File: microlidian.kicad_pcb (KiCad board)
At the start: 2 copper layers, 148.7 x 128.5 mm, 31 parts, among them J1 Conn_02x05_Odd_Even, J11 Backboard Conn 1, J12 Frontboard Conn 1, J13 Backboard Conn 2, J14 Frontboard Conn 2, J2 ST7789 TFT socket, J3 Expansion header, J4 ADS1015 digital side, J5 ADS1015 analog side, J7 TRS MIDI Out, SW1 RotaryEncoder_Switch, SW2 Back button, U1 SeeeduinoXIAO, U2 L78L05_TO92

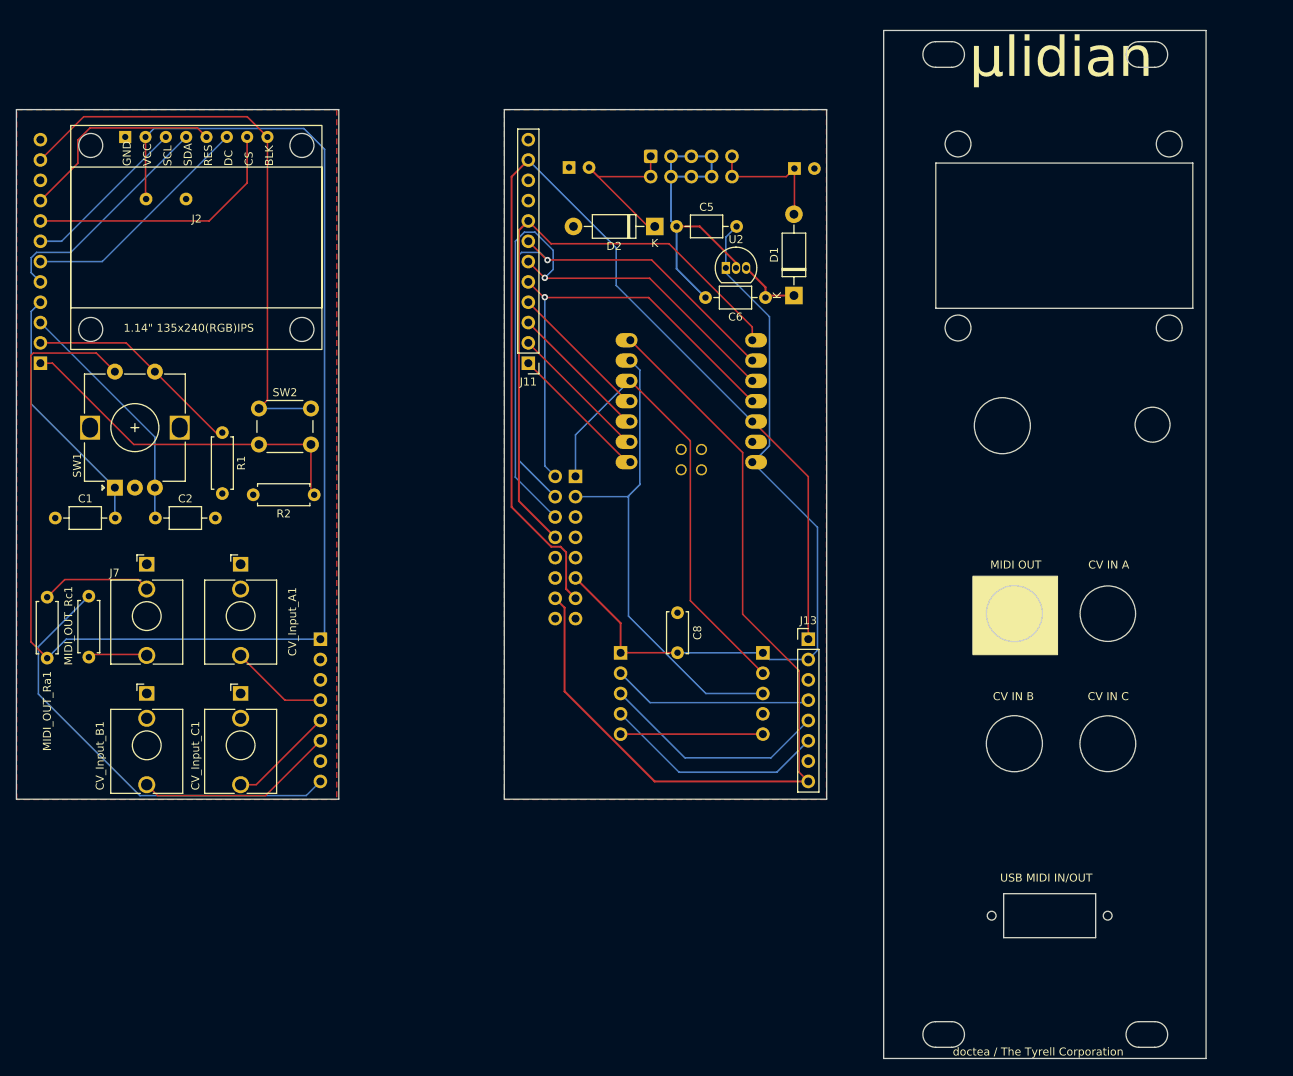
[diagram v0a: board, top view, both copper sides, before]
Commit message: some minor updates
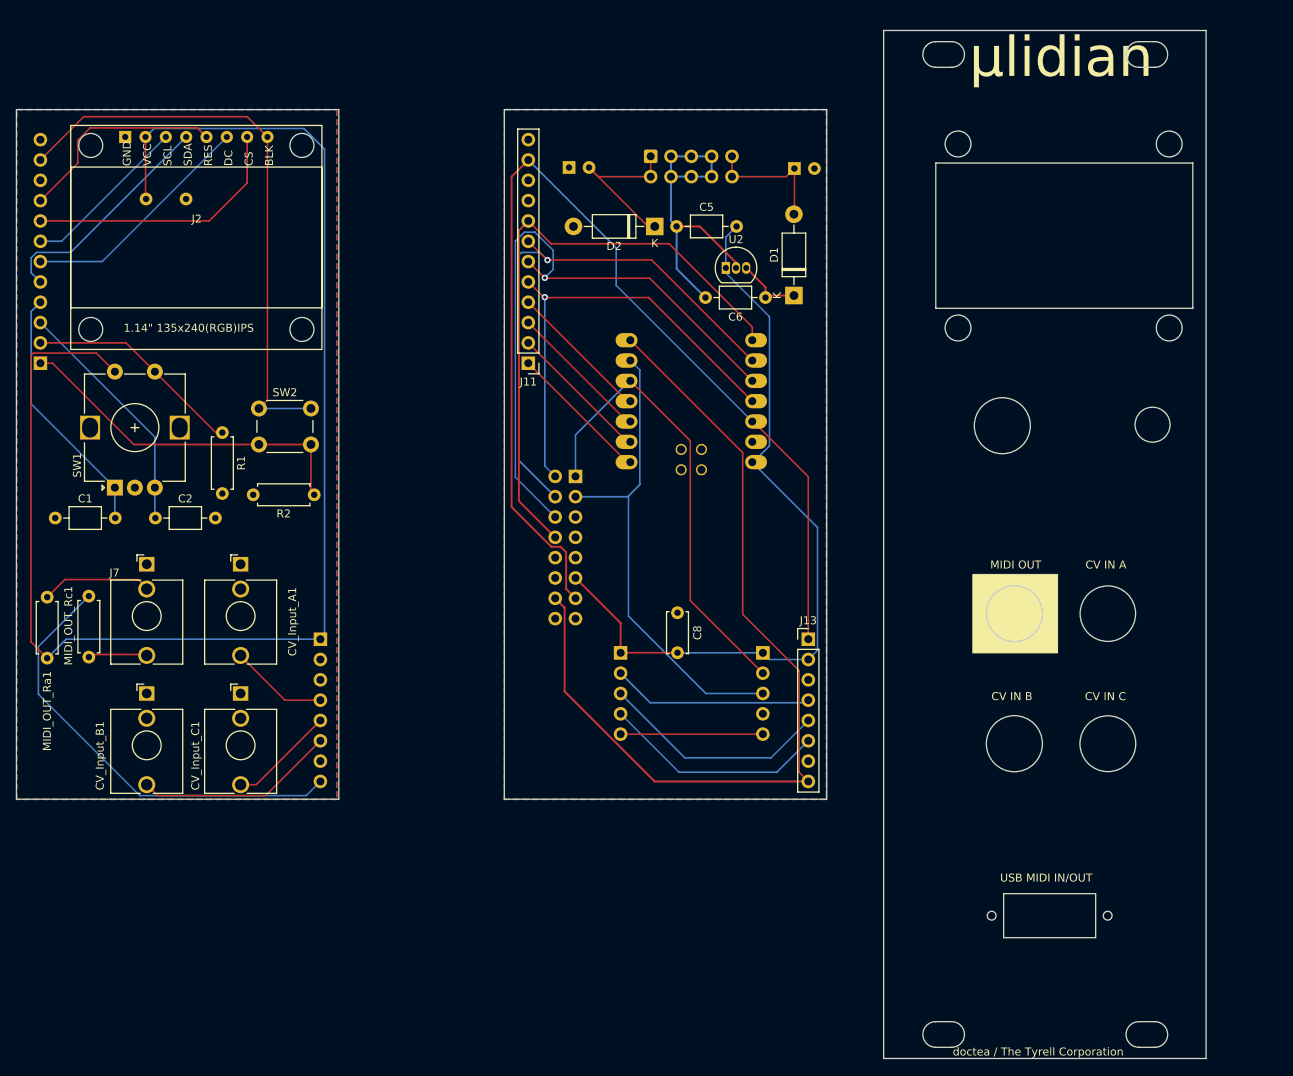
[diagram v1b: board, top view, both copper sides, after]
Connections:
- C1 pad 1: CV GND -> GND
- C2 pad 2: CV GND -> GND
- C3 pad 1: CV GND -> GND
- C4 pad 2: CV GND -> GND
- C5 pad 1: CV GND -> GND
- C6 pad 2: CV GND -> GND
- C7 pad 2: CV GND -> GND
- C8 pad 1: CV GND -> GND
- CV_Input_A1 pad S: CV GND -> GND
- CV_Input_A1 pad TN: CV GND -> GND
- CV_Input_B1 pad S: CV GND -> GND
- CV_Input_B1 pad TN: CV GND -> GND
- CV_Input_C1 pad S: CV GND -> GND
- CV_Input_C1 pad TN: CV GND -> GND
- J1 pad 3: CV GND -> GND
- J1 pad 4: CV GND -> GND
- J1 pad 5: CV GND -> GND
- J1 pad 6: CV GND -> GND
- J1 pad 7: CV GND -> GND
- J1 pad 8: CV GND -> GND
- J11 pad 12: CV GND -> GND
- J12 pad 12: CV GND -> GND
- J13 pad 3: CV GND -> GND
- J13 pad 7: CV GND -> GND
- J14 pad 3: CV GND -> GND
- J14 pad 7: CV GND -> GND
- J2 pad 1: CV GND -> GND
- J3 pad 15: CV GND -> GND
- J3 pad 16: CV GND -> GND
- J4 pad 5: CV GND -> GND
- J7 pad S: CV GND -> GND
- R1 pad 2: CV GND -> GND
- R2 pad 2: CV GND -> GND
- SW1 pad C: CV GND -> GND
- U1 pad 13: CV GND -> GND
- U2 pad 2: CV GND -> GND
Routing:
- net GND: track 0.00 -> 42.1 mm
- net CV GND: track 59.9 -> 17.8 mm
- added copper zone on B.Cu, net GND
- added copper zone on F.Cu, net GND
- removed copper zone on F.Cu, net CV GND
